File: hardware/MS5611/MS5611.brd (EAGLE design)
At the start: 15 x 16 mm, 4 parts, among them U1 MS5611, U2 EM406FLAT

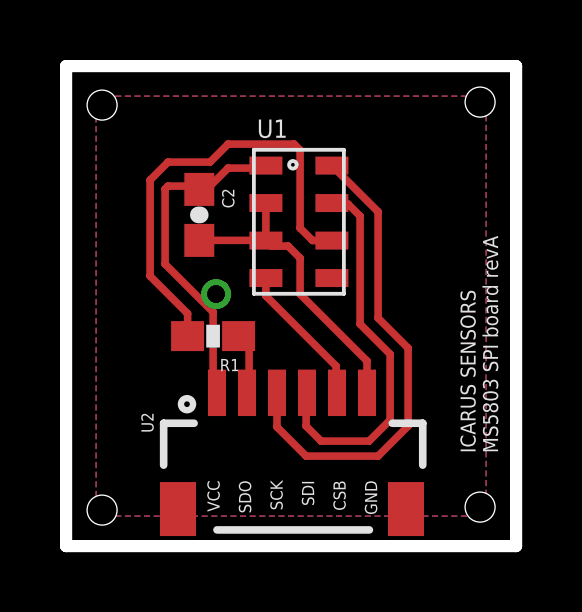
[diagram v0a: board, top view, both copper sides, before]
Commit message: MS5611
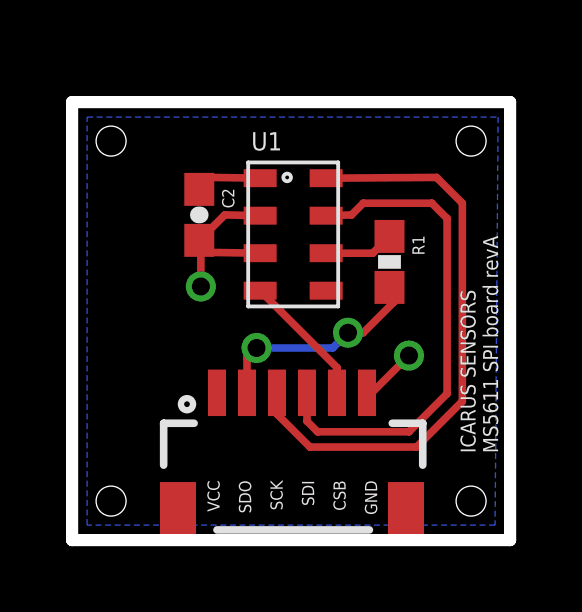
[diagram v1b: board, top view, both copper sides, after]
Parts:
- C2: value 100nF -> 0.1uF
- moved R1 6.38 mm to (10.8, 9.47), turned to 270 degrees
- moved U1 0.46 mm to (7.57, 10.4)
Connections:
- removed net N$6: U1.4, U2.5
- new net N$3: U1.5
- new net VCC: U2.1
- net CSB: now also U1.4, U2.5; no longer U1.5
- net N$1: now also C2.1, U1.1; no longer R1.1, U2.2
- net N$2: now also R1.1, U1.6; no longer C2.1, U1.1, U2.1
- net SDO: now also U2.2; no longer U1.6
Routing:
- net N$2: track 11.5 -> 2.34 mm
- net SDO: track 15.1 -> 7.38 mm, vias 0 -> 2
- net CSB: track 0.00 -> 5.05 mm
- net N$6: track 4.81 -> 0.00 mm
- net SDI: track 12.8 -> 16.5 mm
- net SCK: track 16.1 -> 19.5 mm
- net GND: track 10.3 -> 8.08 mm, vias 1 -> 2
- removed copper zone on layer 1, net GND
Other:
- board size 15 x 16 mm -> 14.6 x 14.6 mm
- board text added: "ICARUS SENSORS MS5611 SPI board revA"
- board text removed: "ICARUS SENSORS MS5803 SPI board revA"
